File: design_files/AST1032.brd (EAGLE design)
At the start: 27 x 23 mm, 12 parts, among them J1 SM05B, J2 OLED

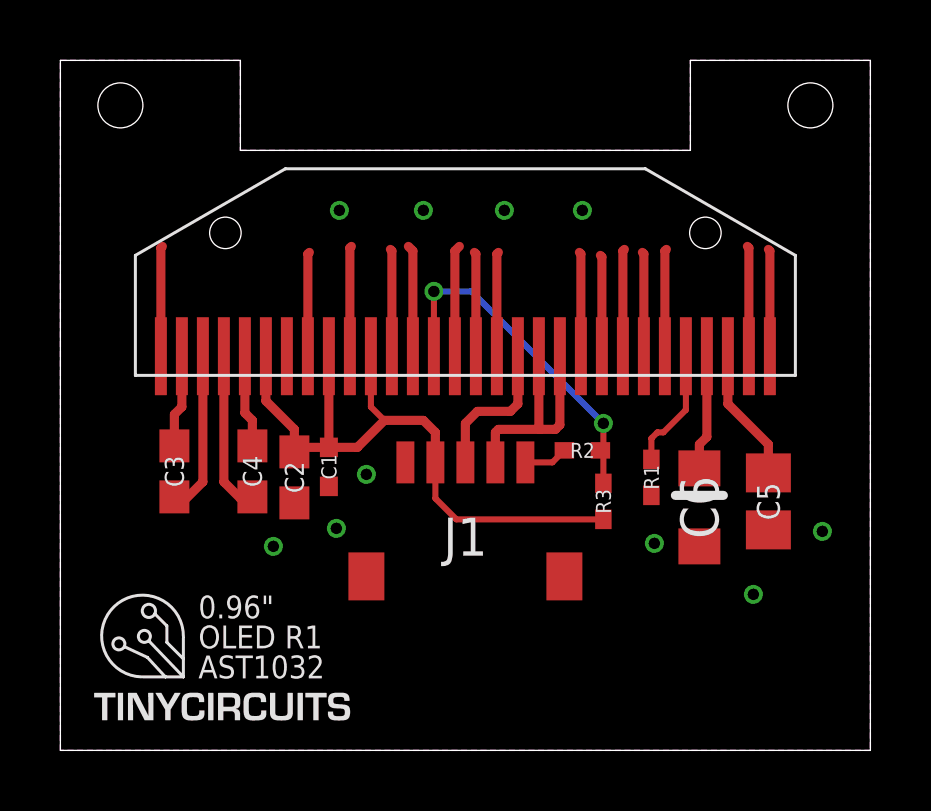
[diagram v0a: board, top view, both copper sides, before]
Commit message: updated documentation
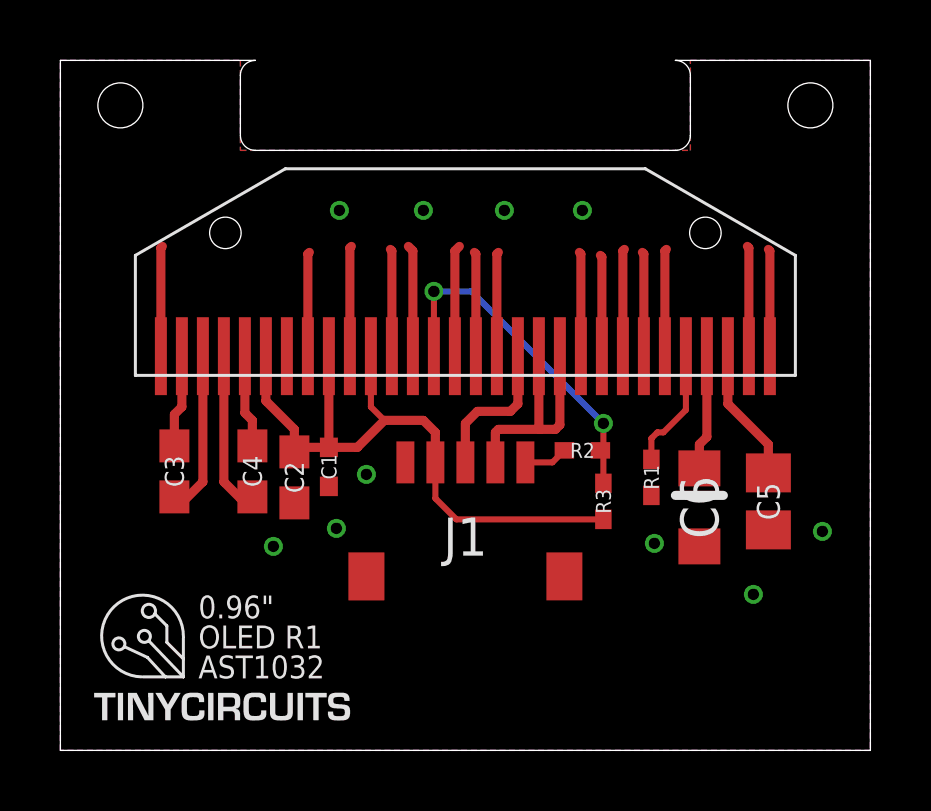
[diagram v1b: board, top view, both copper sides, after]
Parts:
- R2: value 0.0 -> 1.00K
- renumbered J2 to U1
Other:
- outline, holes or cut-outs redrawn
- board text added: "Wireling 0.96 OLED"
- board text removed: "0.96" OLED"
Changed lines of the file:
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@@
 <layer number="59" name="Invisible" color="7" fill="1" visible="no" active="no"/>
 <layer number="61" name="stand" color="7" fill="1" visible="no" active="no"/>
+<layer number="88" name="SimResults" color="9" fill="1" visible="yes" active="yes"/>
+<layer number="89" name="SimProbes" color="9" fill="1" visible="yes" active="yes"/>
 <layer number="90" name="Modules" color="5" fill="1" visible="yes" active="yes"/>
 <layer number="91" name="Nets" color="2" fill="1" visible="no" active="no"/>
@@
 <layer number="158" name="bResistor" color="7" fill="1" visible="no" active="yes"/>
 <layer number="159" name="henwayCAP" color="13" fill="1" visible="yes" active="yes"/>
+<layer number="160" name="IDFDebug" color="7" fill="1" visible="yes" active="yes"/>
 <layer number="191" name="mNets" color="7" fill="1" visible="no" active="no"/>
 <layer number="192" name="mBusses" color="7" fill="1" visible="no" active="no"/>
@@
 <wire x1="0" y1="45.8" x2="0" y2="0" width="0.127" layer="48"/>
 <dimension x1="10" y1="33" x2="37" y2="33" x3="23.5" y3="35.45465" layer="48"/>
-<text x="51.111025" y="4.365003125" size="0.889" layer="48">0.96" OLED</text>
+<text x="51.111025" y="4.365003125" size="0.889" layer="48">Wireling 0.96 OLED</text>
 <text x="47.986825" y="1.7714" size="0.889" layer="48">AS-PCB-AST1032</text>
 <text x="70.3810375" y="1.6952" size="0.889" layer="48">1</text>
@@
 <wire x1="10" y1="33" x2="10" y2="10" width="0.0254" layer="20"/>
 <dimension x1="10" y1="33" x2="10" y2="10" x3="7" y3="21.5" layer="48"/>
-<wire x1="37" y1="33" x2="31" y2="33" width="0.0254" layer="20"/>
-<wire x1="31" y1="33" x2="31" y2="30" width="0.0254" layer="20"/>
-<wire x1="31" y1="30" x2="16" y2="30" width="0.0254" layer="20"/>
-<wire x1="16" y1="30" x2="16" y2="33" width="0.0254" layer="20"/>
-<wire x1="16" y1="33" x2="10" y2="33" width="0.0254" layer="20"/>
+<wire x1="37" y1="33" x2="30.5" y2="33" width="0.0254" layer="20"/>
+<wire x1="31" y1="32.5" x2="31" y2="30.5" width="0.0254" layer="20"/>
+<wire x1="30.5" y1="30" x2="16.5" y2="30" width="0.0254" layer="20"/>
+<wire x1="16.5" y1="30" x2="16" y2="30.5" width="0.0254" layer="20" curve="-90"/>
+<wire x1="16" y1="30.5" x2="16" y2="32.5" width="0.0254" layer="20"/>
+<wire x1="16.5" y1="33" x2="10" y2="33" width="0.0254" layer="20"/>
 <text x="43.0812" y="14.456396875" size="0.4572" layer="48" ratio="10">Released under the Creative Commons Attribution Share-Alike 3.0 License</text>
 <text x="43.0812" y="13.795996875" size="0.4572" layer="48" ratio="10">http://creativecommons.org/licenses/by-sa/3.0</text>
@@
 <text x="14.6" y="12.4" size="0.762" layer="21" rot="SR0">AST1032</text>
 <rectangle x1="12.9" y1="21.5" x2="34.1" y2="26.3" layer="41"/>
+<wire x1="16" y1="32.5" x2="16.5" y2="33" width="0.0254" layer="20" curve="-90"/>
+<wire x1="31" y1="30.5" x2="30.5" y2="30" width="0.0254" layer="20" curve="-90"/>
+<wire x1="30.5" y1="33" x2="31" y2="32.5" width="0.0254" layer="20" curve="-90"/>
 </plain>
 <attributes>
@@
 <attribute name="PNPROTATION" value="180" x="23.5" y="17.125" size="1.778" layer="27" display="off"/>
 </element>
-<element name="J2" library="tinycircuits" package="OLED_WHITE_30P" value="OLED" x="23.5" y="25.5">
+<element name="U1" library="tinycircuits" package="OLED_WHITE_30P" value="OLED" x="23.5" y="25.5">
 <attribute name="PARTNO" value="AS-ITM-00341" x="23.5" y="25.5" size="1.778" layer="27" display="off"/>
 <attribute name="VALUE" value="OLED" x="23.5" y="25.5" size="1.778" layer="27" display="off"/>
@@
 <attribute name="VALUE" value="390K" x="29.7" y="19.1" size="1.778" layer="27" rot="R90" display="off"/>
 </element>
-<element name="R2" library="tinycircuits" package="0402" value="0.0" x="27.4" y="20">
-<attribute name="PARTNO" value="AS-ITM-00076" x="27.4" y="20" size="1.778" layer="27" display="off"/>
-<attribute name="VALUE" value="0.0" x="27.4" y="20" size="1.778" layer="27" display="off"/>
+<element name="R2" library="tinycircuits" package="0402" value="1.00K" x="27.4" y="20">
+<attribute name="PARTNO" value="AS-ITM-00003" x="27.4" y="20" size="1.778" layer="27" display="off"/>
+<attribute name="VALUE" value="1.00K" x="27.4" y="20" size="1.778" layer="27" display="off"/>
 </element>
 <element name="C5" library="tinycircuits" package="C0805" value="10uF" x="33.6" y="18.3" rot="R270">
@@
 <via x="17.1" y="16.8" extent="1-16" drill="0.381"/>
 <contactref element="R1" pad="1"/>
-<contactref element="J2" pad="1"/>
-<contactref element="J2" pad="2"/>
-<contactref element="J2" pad="6"/>
-<contactref element="J2" pad="10"/>
-<contactref element="J2" pad="9"/>
-<contactref element="J2" pad="8"/>
-<contactref element="J2" pad="7"/>
-<contactref element="J2" pad="30"/>
-<contactref element="J2" pad="21"/>
-<contactref element="J2" pad="19"/>
-<contactref element="J2" pad="18"/>
-<contactref element="J2" pad="16"/>
-<contactref element="J2" pad="15"/>
-<contactref element="J2" pad="14"/>
+<contactref element="U1" pad="1"/>
+<contactref element="U1" pad="2"/>
+<contactref element="U1" pad="6"/>
+<contactref element="U1" pad="10"/>
+<contactref element="U1" pad="9"/>
+<contactref element="U1" pad="8"/>
+<contactref element="U1" pad="7"/>
+<contactref element="U1" pad="30"/>
+<contactref element="U1" pad="21"/>
+<contactref element="U1" pad="19"/>
+<contactref element="U1" pad="18"/>
+<contactref element="U1" pad="16"/>
+<contactref element="U1" pad="15"/>
+<contactref element="U1" pad="14"/>
 <contactref element="C5" pad="2"/>
 <contactref element="C6" pad="2"/>
-<contactref element="J2" pad="23"/>
+<contactref element="U1" pad="23"/>
 <via x="20.2" y="19.2" extent="1-16" drill="0.381"/>
 <via x="29.8" y="16.9" extent="1-16" drill="0.381"/>
@@
 <signal name="SDA">
 <contactref element="J1" pad="4"/>
-<contactref element="J2" pad="12"/>
-<contactref element="J2" pad="11"/>
+<contactref element="U1" pad="12"/>
+<contactref element="U1" pad="11"/>
 <wire x1="25.95" y1="23.14" x2="25.95" y2="20.75" width="0.3048" layer="1"/>
 <wire x1="25.95" y1="20.75" x2="26" y2="20.7" width="0.3048" layer="1"/>
@@
 <signal name="SCL">
 <contactref element="J1" pad="3"/>
-<contactref element="J2" pad="13"/>
+<contactref element="U1" pad="13"/>
 <wire x1="25.25" y1="23.14" x2="25.25" y2="21.55" width="0.3048" layer="1"/>
 <wire x1="25.25" y1="21.55" x2="25" y2="21.3" width="0.3048" layer="1"/>
@@
 <contactref element="C2" pad="1"/>
 <contactref element="J1" pad="2"/>
-<contactref element="J2" pad="25"/>
-<contactref element="J2" pad="22"/>
-<contactref element="J2" pad="20"/>
+<contactref element="U1" pad="25"/>
+<contactref element="U1" pad="22"/>
+<contactref element="U1" pad="20"/>
 <contactref element="R3" pad="2"/>
 <wire x1="22.5" y1="19.6" x2="22.5" y2="20.6" width="0.3048" layer="1"/>
@@
 </signal>
 <signal name="N$1">
-<contactref element="J2" pad="29"/>
+<contactref element="U1" pad="29"/>
 <contactref element="C3" pad="1"/>
 <wire x1="14.05" y1="23.14" x2="14.05" y2="21.45" width="0.3048" layer="1"/>
@@
 </signal>
 <signal name="N$2">
-<contactref element="J2" pad="28"/>
+<contactref element="U1" pad="28"/>
 <contactref element="C3" pad="2"/>
 <wire x1="14.75" y1="23.14" x2="14.75" y2="18.95" width="0.3048" layer="1"/>
@@
 </signal>
 <signal name="N$4">
-<contactref element="J2" pad="27"/>
+<contactref element="U1" pad="27"/>
 <contactref element="C4" pad="1"/>
 <wire x1="15.45" y1="23.14" x2="15.45" y2="18.95" width="0.3048" layer="1"/>
@@
 <signal name="N$5">
 <contactref element="C4" pad="2"/>
-<contactref element="J2" pad="26"/>
+<contactref element="U1" pad="26"/>
 <wire x1="16.15" y1="23.14" x2="16.15" y2="21.25" width="0.3048" layer="1"/>
 <wire x1="16.15" y1="21.25" x2="16.4" y2="21" width="0.3048" layer="1"/>
@@
 <signal name="N$7">
 <contactref element="R1" pad="2"/>
-<contactref element="J2" pad="5"/>
+<contactref element="U1" pad="5"/>
 <wire x1="30.85" y1="23.14" x2="30.85" y2="21.35" width="0.2032" layer="1"/>
 <wire x1="30.85" y1="21.35" x2="30.1" y2="20.6" width="0.2032" layer="1"/>
@@
 </signal>
 <signal name="N$3">
-<contactref element="J2" pad="4"/>
+<contactref element="U1" pad="4"/>
 <contactref element="C6" pad="1"/>
 <wire x1="31.55" y1="23.14" x2="31.55" y2="20.45" width="0.3048" layer="1"/>
@@
 </signal>
 <signal name="N$8">
-<contactref element="J2" pad="3"/>
+<contactref element="U1" pad="3"/>
 <contactref element="C5" pad="1"/>
 <wire x1="32.25" y1="23.14" x2="32.25" y2="21.55" width="0.3048" layer="1"/>
@@
 </signal>
 <signal name="N$9">
-<contactref element="J2" pad="17"/>
+<contactref element="U1" pad="17"/>
 <contactref element="R2" pad="2"/>
 <contactref element="R3" pad="1"/>
